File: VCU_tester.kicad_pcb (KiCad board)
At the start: 2 copper layers, 200 x 159 mm, 125 parts, among them J1 Conn_01x04_Male, J10 DB9_Male, J11 DB9_Male, J12 Conn_01x08_Male, J13 Conn_01x08_Male, J14 USB_C_Receptacle, J15 USB_B_Micro, J16 Conn_01x05_Male, J2 Screw_Terminal_01x02, J3 DB9_Male, J4 DB9_Male, J5 DB9_Male, J500 Conn_01x10_Female, J501 Conn_01x08_Female, J502 Conn_01x08_Female, J503 Conn_01x08_Female, J504 Conn_01x08_Female, J505 Conn_01x08_Female, J507 Conn_02x18_Odd_Even, J6 DB9_Male, J7 Conn_01x04_Male, J8 DB9_Male, J9 DB9_Male, P8 BeagleBone_Black_Header, P9 BeagleBone_Black_Header, U1 REF3020, U2 MAX3232, U3 TCAN1042HVD, U4 MAX3232, U5 TCAN1042HVD, U6 DS3231MZ, U7 DS3231MZ

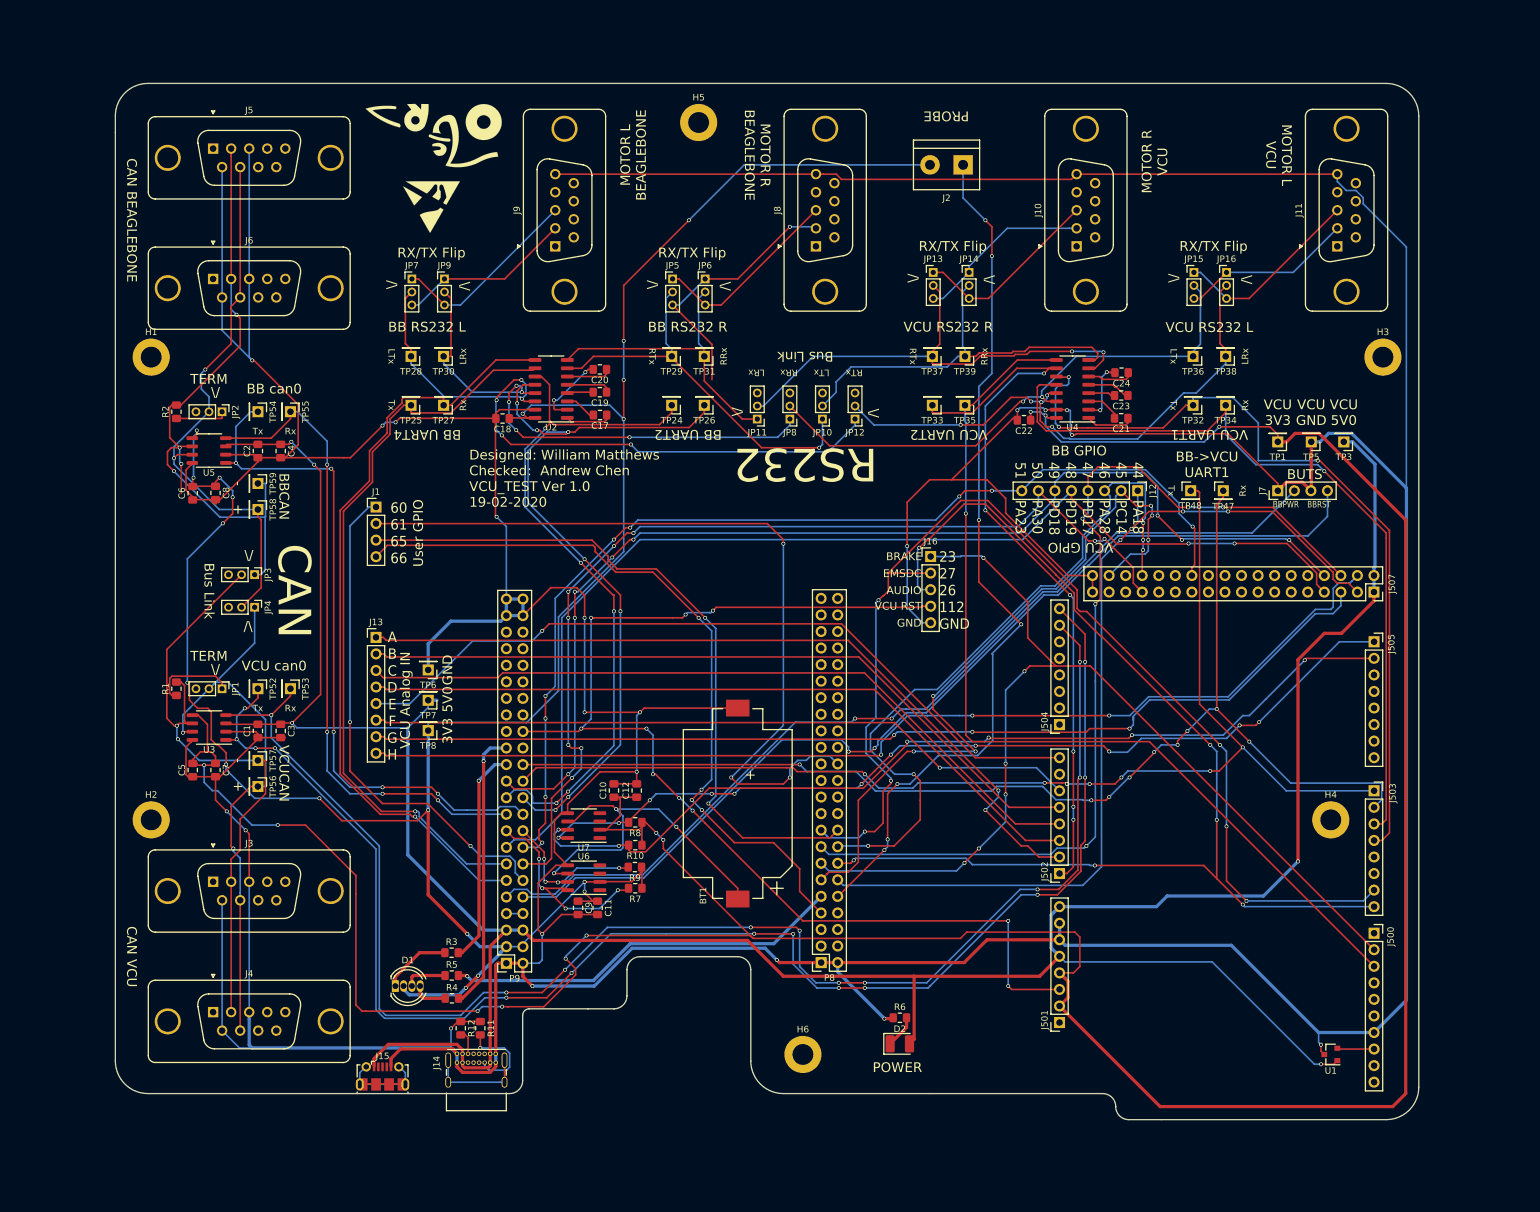
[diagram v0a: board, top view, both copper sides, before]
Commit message: ground plane, checked, ready to go?
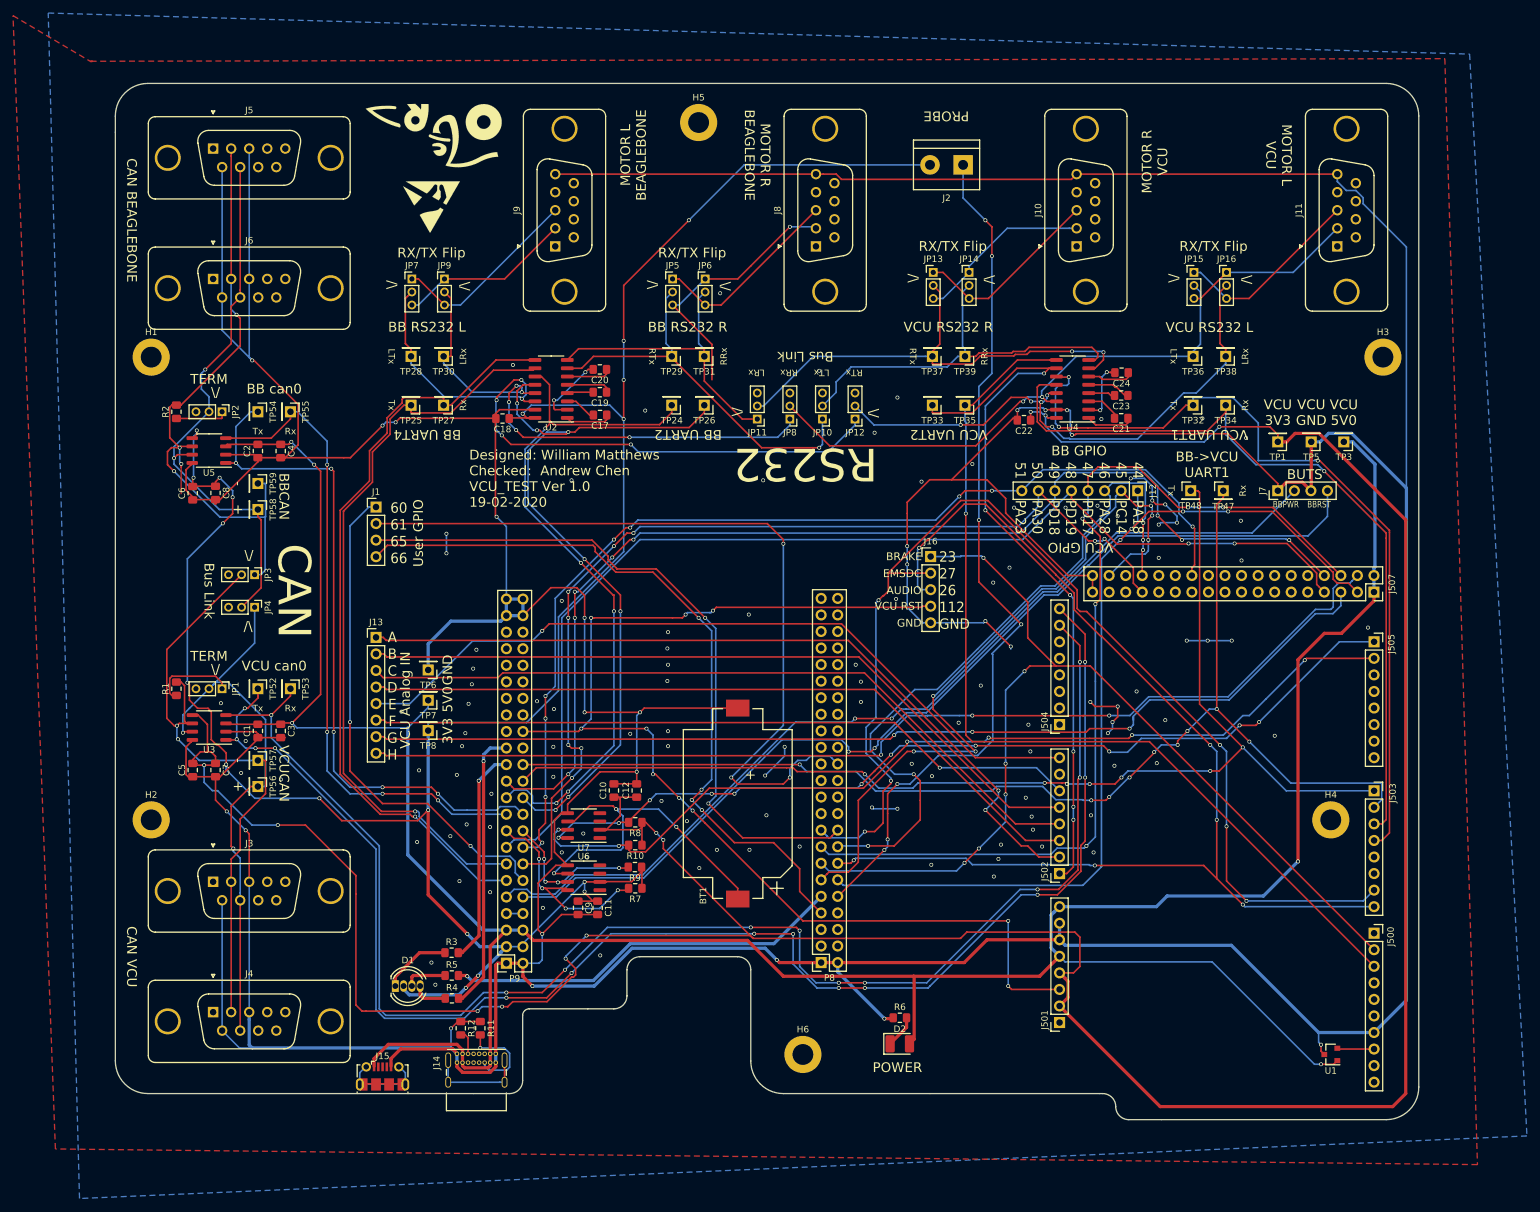
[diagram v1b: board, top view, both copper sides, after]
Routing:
- net GNDD: track 1094.2 -> 1152.1 mm, vias 21 -> 137
- net +5V: track 447.9 -> 446.6 mm
- added copper zone on B.Cu, net GNDD
- added copper zone on F.Cu, net GNDD
